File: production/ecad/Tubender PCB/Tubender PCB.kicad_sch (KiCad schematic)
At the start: 0 parts

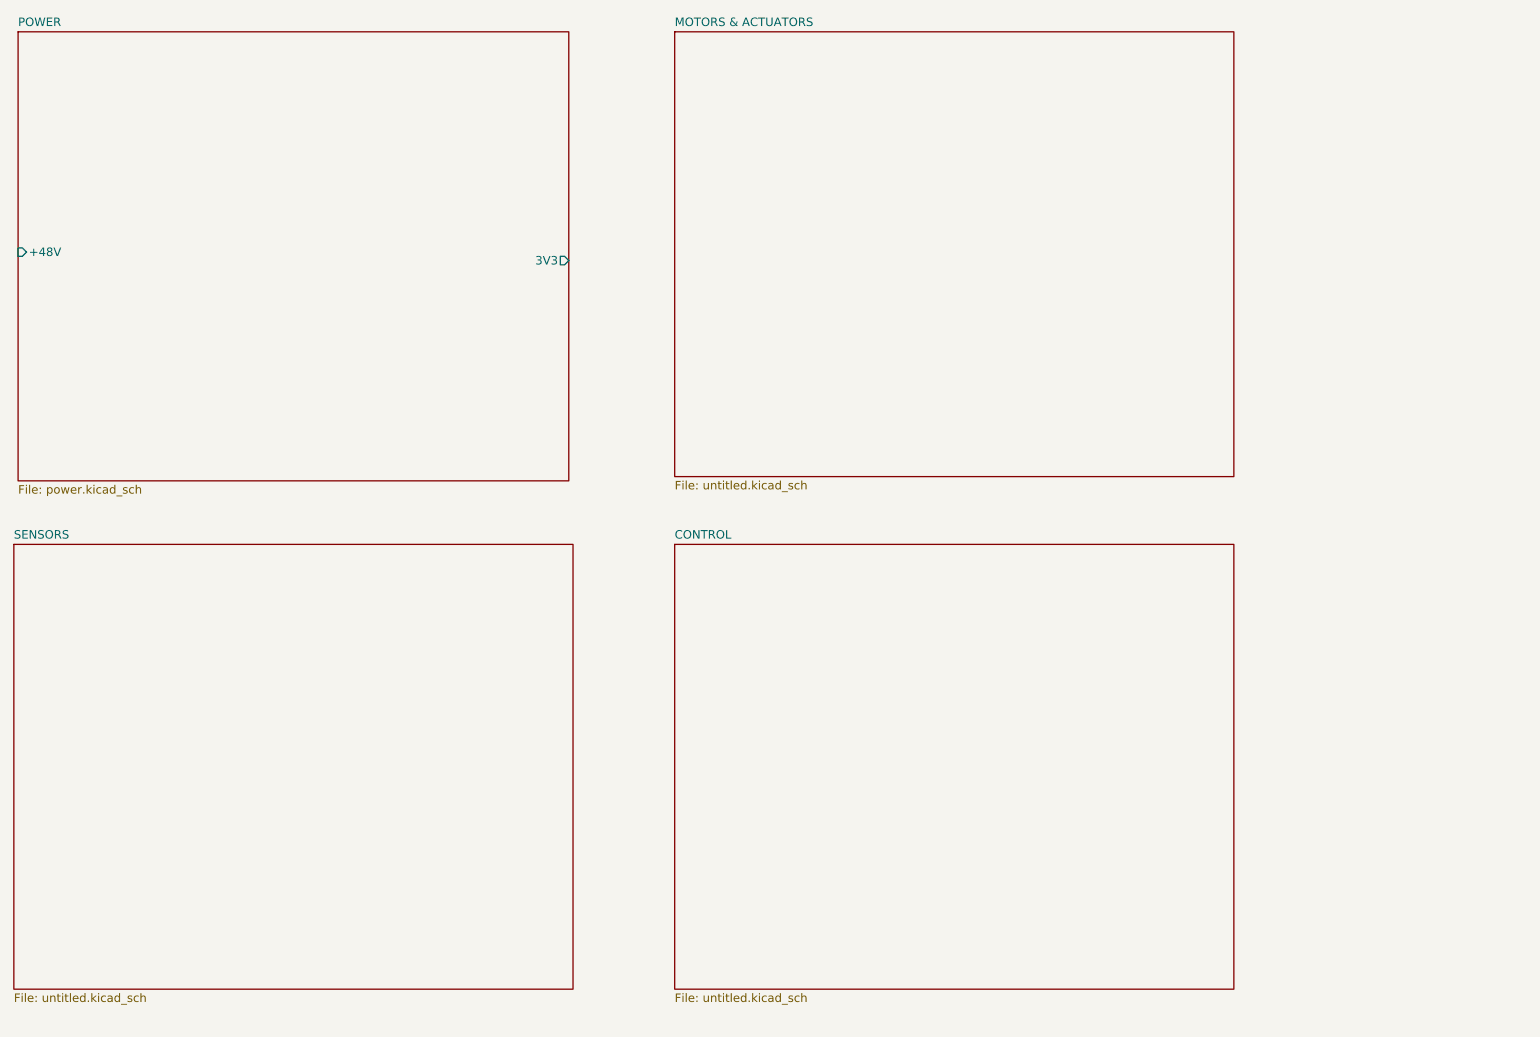
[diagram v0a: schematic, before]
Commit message: MCU and such
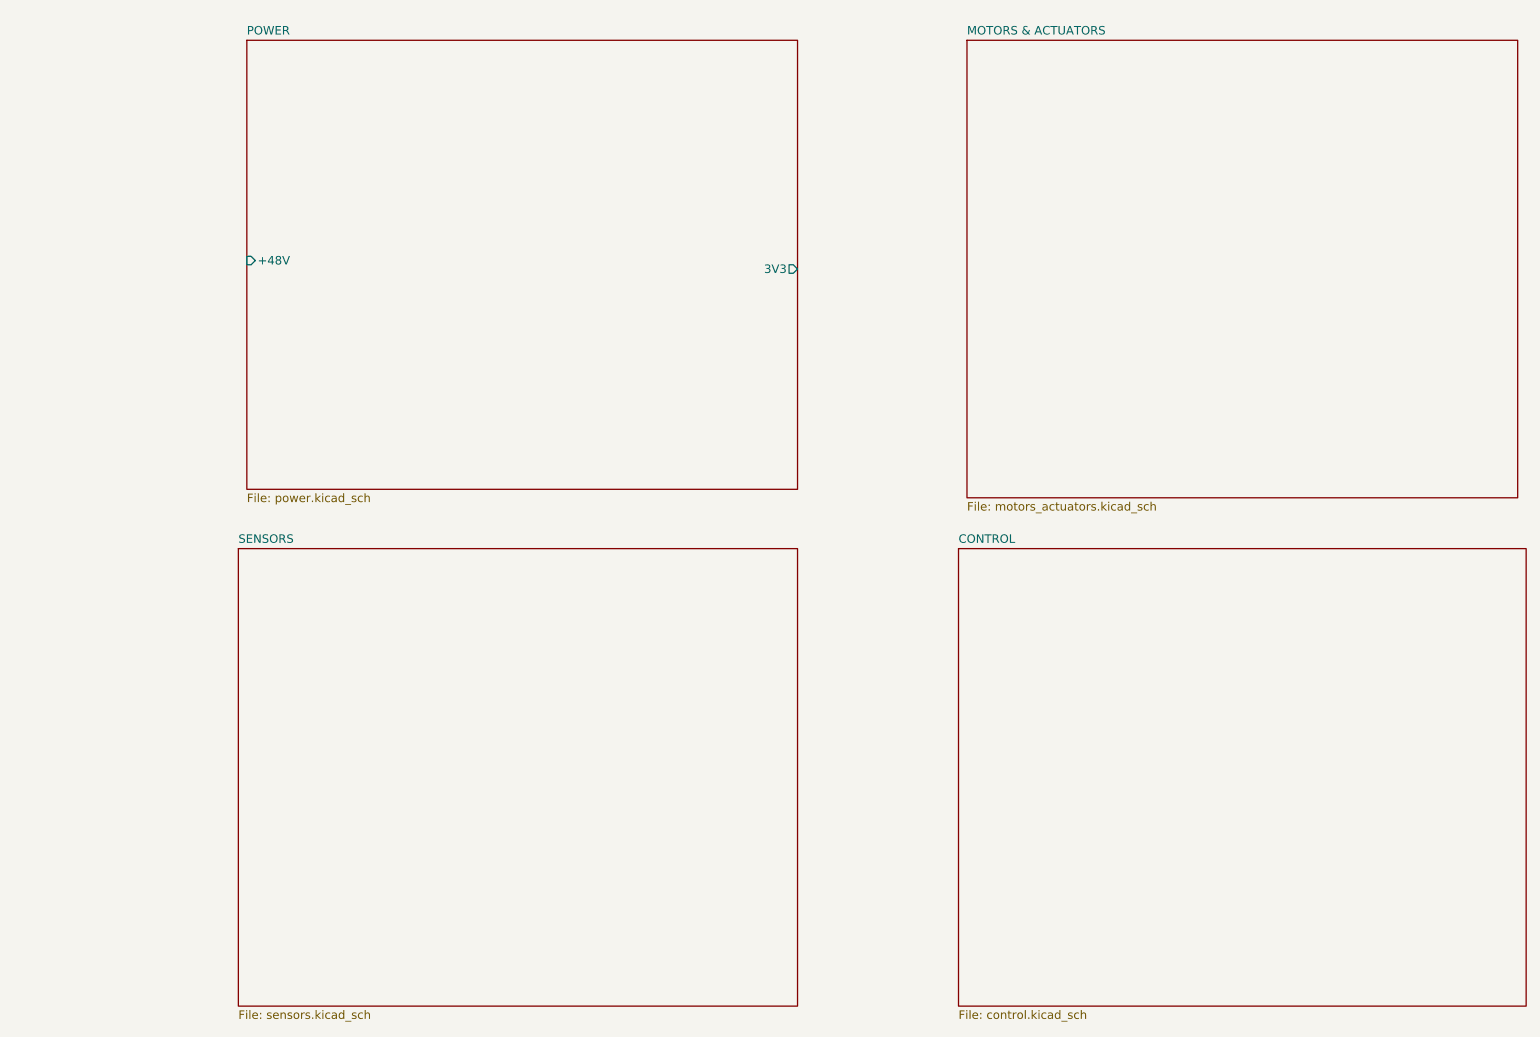
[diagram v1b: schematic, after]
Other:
- sheet CONTROL: file untitled.kicad_sch -> control.kicad_sch
- sheet MOTORS & ACTUATORS: file untitled.kicad_sch -> motors_actuators.kicad_sch
- sheet SENSORS: file untitled.kicad_sch -> sensors.kicad_sch
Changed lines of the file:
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@@
 	)
 	(sheet
-		(at 17.78 16.51)
+		(at 160.02 17.78)
+		(size 82.55 68.58)
+		(fields_autoplaced yes)
+		(stroke
+			(width 0.1524)
+			(type solid)
+		)
+		(fill
+			(color 0 0 0 0.0000)
+		)
+		(property "Sheetname" "MOTORS & ACTUATORS"
+			(at 160.02 17.0684 0)
+			(effects
+				(font
+					(size 1.27 1.27)
+				)
+				(justify left bottom)
+			)
+		)
+		(property "Sheetfile" "motors_actuators.kicad_sch"
+			(at 160.02 86.9446 0)
+			(effects
+				(font
+					(size 1.27 1.27)
+				)
+				(justify left top)
+			)
+		)
+		(instances
+			(project "Tubender PCB"
+				(path "/3e1aedd0-6089-4edb-92c7-0c31da2e7927"
+					(page "3")
+				)
+			)
+		)
+	)
+	(sheet
+		(at 52.07 17.78)
 		(size 82.55 67.31)
 		(fields_autoplaced yes)
@@
 		)
 		(property "Sheetname" "POWER"
-			(at 17.78 15.7984 0)
+			(at 52.07 17.0684 0)
 			(effects
 				(font
@@
 		)
 		(property "Sheetfile" "power.kicad_sch"
-			(at 17.78 84.4046 0)
+			(at 52.07 85.6746 0)
 			(effects
 				(font
@@
 		)
 		(pin "3V3" output
-			(at 100.33 50.8 0)
+			(at 134.62 52.07 0)
 			(effects
 				(font
@@
 		)
 		(pin "+48V" input
-			(at 17.78 49.53 180)
+			(at 52.07 50.8 180)
 			(effects
 				(font
@@
 	)
 	(sheet
-		(at 17.145 93.345)
-		(size 83.82 66.675)
-		(fields_autoplaced yes)
-		(stroke
-			(width 0.1524)
-			(type solid)
-		)
-		(fill
-			(color 0 0 0 0.0000)
-		)
-		(property "Sheetname" "SENSORS"
-			(at 17.145 92.6334 0)
-			(effects
-				(font
-					(size 1.27 1.27)
-				)
-				(justify left bottom)
-			)
-		)
-		(property "Sheetfile" "untitled.kicad_sch"
-			(at 17.145 160.6046 0)
-			(effects
-				(font
-					(size 1.27 1.27)
-				)
-				(justify left top)
-			)
-		)
-		(instances
-			(project "Tubender PCB"
-				(path "/3e1aedd0-6089-4edb-92c7-0c31da2e7927"
-					(page "3")
-				)
-			)
-		)
-	)
-	(sheet
-		(at 116.205 93.345)
-		(size 83.82 66.675)
+		(at 158.75 93.98)
+		(size 85.09 68.58)
 		(fields_autoplaced yes)
 		(stroke
@@
 		)
 		(property "Sheetname" "CONTROL"
-			(at 116.205 92.6334 0)
+			(at 158.75 93.2684 0)
 			(effects
 				(font
@@
 			)
 		)
-		(property "Sheetfile" "untitled.kicad_sch"
-			(at 116.205 160.6046 0)
+		(property "Sheetfile" "control.kicad_sch"
+			(at 158.75 163.1446 0)
 			(effects
 				(font
@@
 	)
 	(sheet
-		(at 116.205 16.51)
-		(size 83.82 66.675)
+		(at 50.8 93.98)
+		(size 83.82 68.58)
 		(fields_autoplaced yes)
 		(stroke
@@
 			(color 0 0 0 0.0000)
 		)
-		(property "Sheetname" "MOTORS & ACTUATORS"
-			(at 116.205 15.7984 0)
+		(property "Sheetname" "SENSORS"
+			(at 50.8 93.2684 0)
 			(effects
 				(font
@@
 			)
 		)
-		(property "Sheetfile" "untitled.kicad_sch"
-			(at 116.205 83.7696 0)
+		(property "Sheetfile" "sensors.kicad_sch"
+			(at 50.8 163.1446 0)
 			(effects
 				(font
